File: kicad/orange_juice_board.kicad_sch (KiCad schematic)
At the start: 63 parts, among them J10 PWM_OUT1, J11 CONN_UART, J12 Conn_01x08, J12 PWM_OUT2, J13 FAN_12/24v, J15 PWM_OUT3, J2 DC_INPUT, J3 CONN_ADXL345, J4 OrangePi Zero GPIO PINs, J7 OrangePi Zero Function Interf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, J8 FAN_5v, J9 PWR_5v, Q1 AO4407A, Q2 AO3400A, Q3 AO3400A, Q4 AO3400A, U1 MP2315GJ-Z

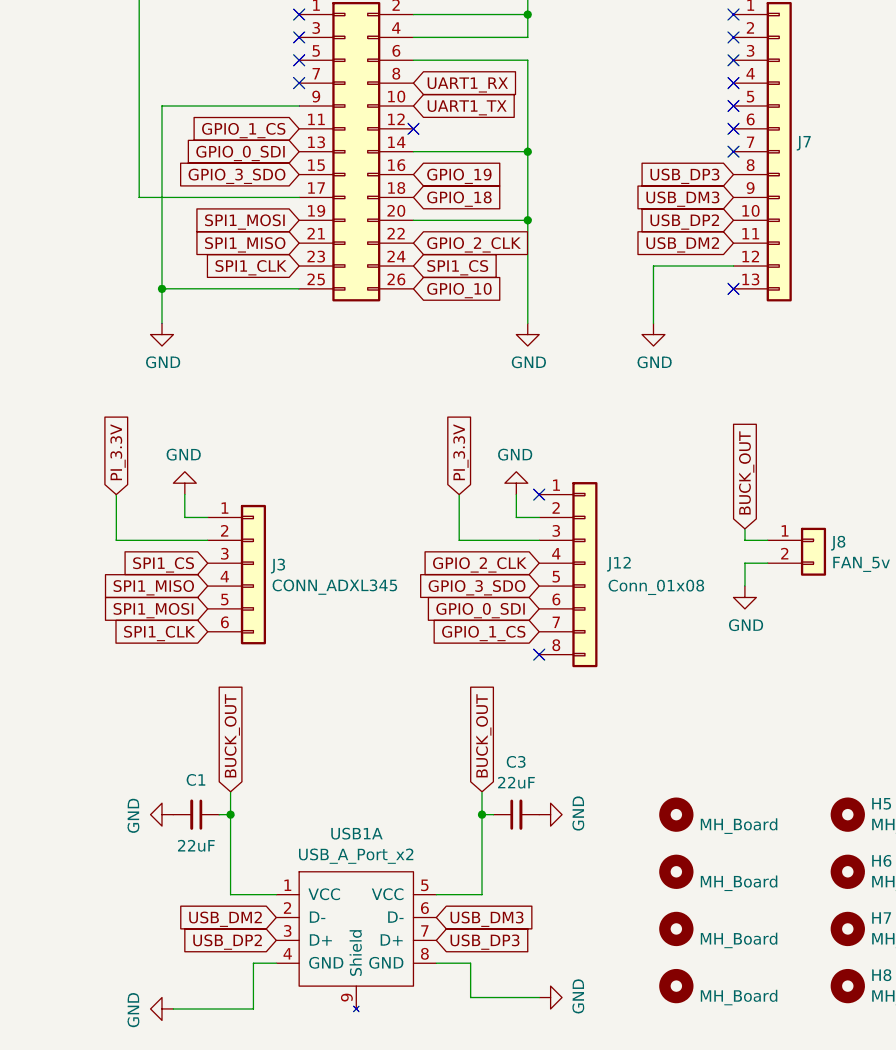
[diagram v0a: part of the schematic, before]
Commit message: update to v0.7
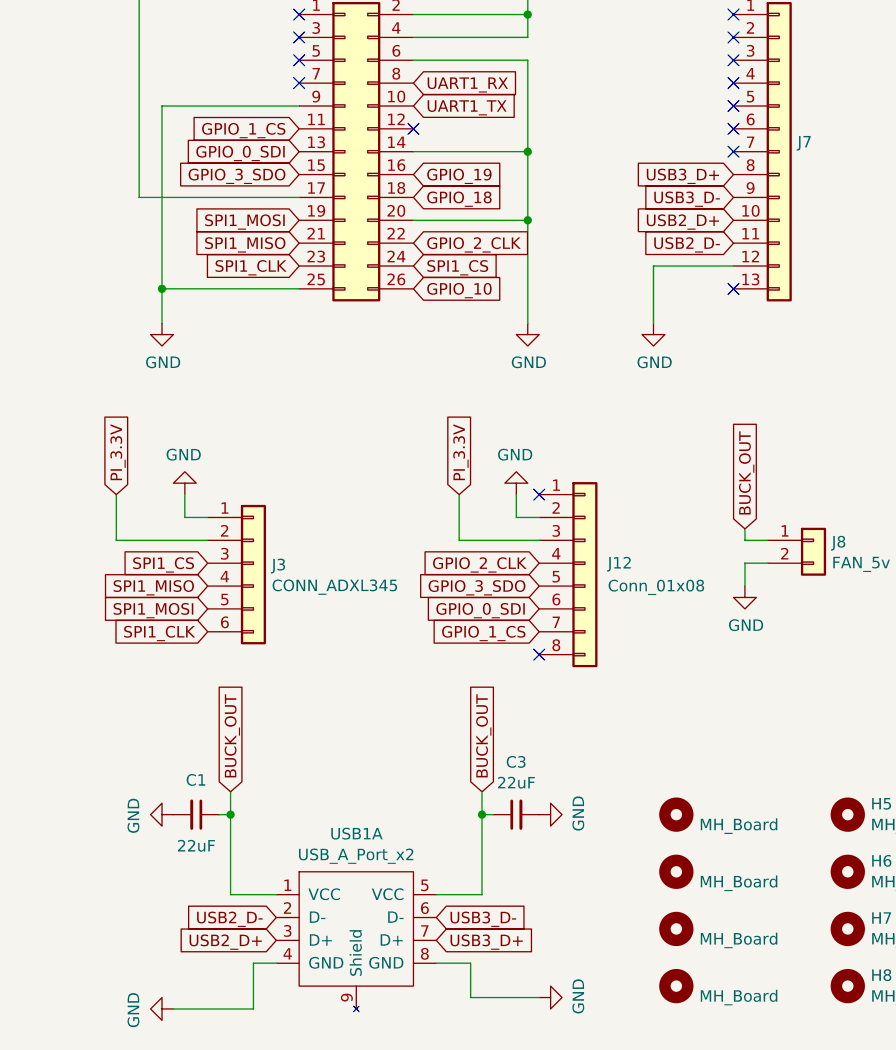
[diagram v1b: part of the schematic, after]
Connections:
- net USB_DM2 renamed USB2_D-
- net USB_DM3 renamed USB3_D-
- net USB_DP2 renamed USB2_D+
- net USB_DP3 renamed USB3_D+
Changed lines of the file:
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@@
     )
   )
-  (global_label "USB_DM2" (shape input) (at 95.25 101.6 180) (fields_autoplaced)
-    (effects (font (size 1.27 1.27)) (justify right))
-    (property "Intersheet References" "${INTERSHEET_REFS}" (id 0) (at -8.89 0 0)
-      (effects (font (size 1.27 1.27)) hide)
+  (global_label "USB2_D-" (shape input) (at 95.25 101.6 180) (fields_autoplaced)
+    (effects (font (size 1.27 1.27)) (justify right))
+    (property "Intersheet References" "${INTERSHEET_REFS}" (id 0) (at 84.0963 101.5206 0)
+      (effects (font (size 1.27 1.27)) (justify right) hide)
     )
   )
@@
     )
   )
-  (global_label "USB_DM3" (shape input) (at 62.23 176.53 0) (fields_autoplaced)
-    (effects (font (size 1.27 1.27)) (justify left))
-    (property "Intersheet References" "${INTERSHEET_REFS}" (id 0) (at 33.02 0 0)
-      (effects (font (size 1.27 1.27)) hide)
+  (global_label "USB3_D-" (shape input) (at 62.23 176.53 0) (fields_autoplaced)
+    (effects (font (size 1.27 1.27)) (justify left))
+    (property "Intersheet References" "${INTERSHEET_REFS}" (id 0) (at 73.3837 176.4506 0)
+      (effects (font (size 1.27 1.27)) (justify left) hide)
     )
   )
@@
     )
   )
-  (global_label "USB_DM2" (shape input) (at 44.45 176.53 180) (fields_autoplaced)
-    (effects (font (size 1.27 1.27)) (justify right))
-    (property "Intersheet References" "${INTERSHEET_REFS}" (id 0) (at 73.66 345.44 0)
-      (effects (font (size 1.27 1.27)) hide)
+  (global_label "USB2_D-" (shape input) (at 44.45 176.53 180) (fields_autoplaced)
+    (effects (font (size 1.27 1.27)) (justify right))
+    (property "Intersheet References" "${INTERSHEET_REFS}" (id 0) (at 33.2963 176.4506 0)
+      (effects (font (size 1.27 1.27)) (justify right) hide)
     )
   )
@@
     )
   )
-  (global_label "USB_DP2" (shape input) (at 44.45 179.07 180) (fields_autoplaced)
-    (effects (font (size 1.27 1.27)) (justify right))
-    (property "Intersheet References" "${INTERSHEET_REFS}" (id 0) (at 73.66 350.52 0)
-      (effects (font (size 1.27 1.27)) hide)
+  (global_label "USB2_D+" (shape input) (at 44.45 179.07 180) (fields_autoplaced)
+    (effects (font (size 1.27 1.27)) (justify right))
+    (property "Intersheet References" "${INTERSHEET_REFS}" (id 0) (at 33.2963 178.9906 0)
+      (effects (font (size 1.27 1.27)) (justify right) hide)
     )
   )
@@
     )
   )
-  (global_label "USB_DP2" (shape input) (at 95.25 99.06 180) (fields_autoplaced)
-    (effects (font (size 1.27 1.27)) (justify right))
-    (property "Intersheet References" "${INTERSHEET_REFS}" (id 0) (at -8.89 0 0)
-      (effects (font (size 1.27 1.27)) hide)
-    )
-  )
-  (global_label "USB_DP3" (shape input) (at 95.25 93.98 180) (fields_autoplaced)
-    (effects (font (size 1.27 1.27)) (justify right))
-    (property "Intersheet References" "${INTERSHEET_REFS}" (id 0) (at -8.89 0 0)
-      (effects (font (size 1.27 1.27)) hide)
+  (global_label "USB2_D+" (shape input) (at 95.25 99.06 180) (fields_autoplaced)
+    (effects (font (size 1.27 1.27)) (justify right))
+    (property "Intersheet References" "${INTERSHEET_REFS}" (id 0) (at 84.0963 98.9806 0)
+      (effects (font (size 1.27 1.27)) (justify right) hide)
+    )
+  )
+  (global_label "USB3_D+" (shape input) (at 95.25 93.98 180) (fields_autoplaced)
+    (effects (font (size 1.27 1.27)) (justify right))
+    (property "Intersheet References" "${INTERSHEET_REFS}" (id 0) (at 84.0963 93.9006 0)
+      (effects (font (size 1.27 1.27)) (justify right) hide)
     )
   )
@@
     )
   )
-  (global_label "USB_DM3" (shape input) (at 95.25 96.52 180) (fields_autoplaced)
-    (effects (font (size 1.27 1.27)) (justify right))
-    (property "Intersheet References" "${INTERSHEET_REFS}" (id 0) (at -8.89 0 0)
-      (effects (font (size 1.27 1.27)) hide)
+  (global_label "USB3_D-" (shape input) (at 95.25 96.52 180) (fields_autoplaced)
+    (effects (font (size 1.27 1.27)) (justify right))
+    (property "Intersheet References" "${INTERSHEET_REFS}" (id 0) (at 84.0963 96.4406 0)
+      (effects (font (size 1.27 1.27)) (justify right) hide)
     )
   )
@@
     )
   )
-  (global_label "USB_DP3" (shape input) (at 62.23 179.07 0) (fields_autoplaced)
-    (effects (font (size 1.27 1.27)) (justify left))
-    (property "Intersheet References" "${INTERSHEET_REFS}" (id 0) (at 33.02 0 0)
-      (effects (font (size 1.27 1.27)) hide)
-    )
-  )
+  (global_label "USB3_D+" (shape input) (at 62.23 179.07 0) (fields_autoplaced)
+    (effects (font (size 1.27 1.27)) (justify left))
+    (property "Intersheet References" "${INTERSHEET_REFS}" (id 0) (at 73.3837 178.9906 0)
+      (effects (font (size 1.27 1.27)) (justify left) hide)
+    )
+  )

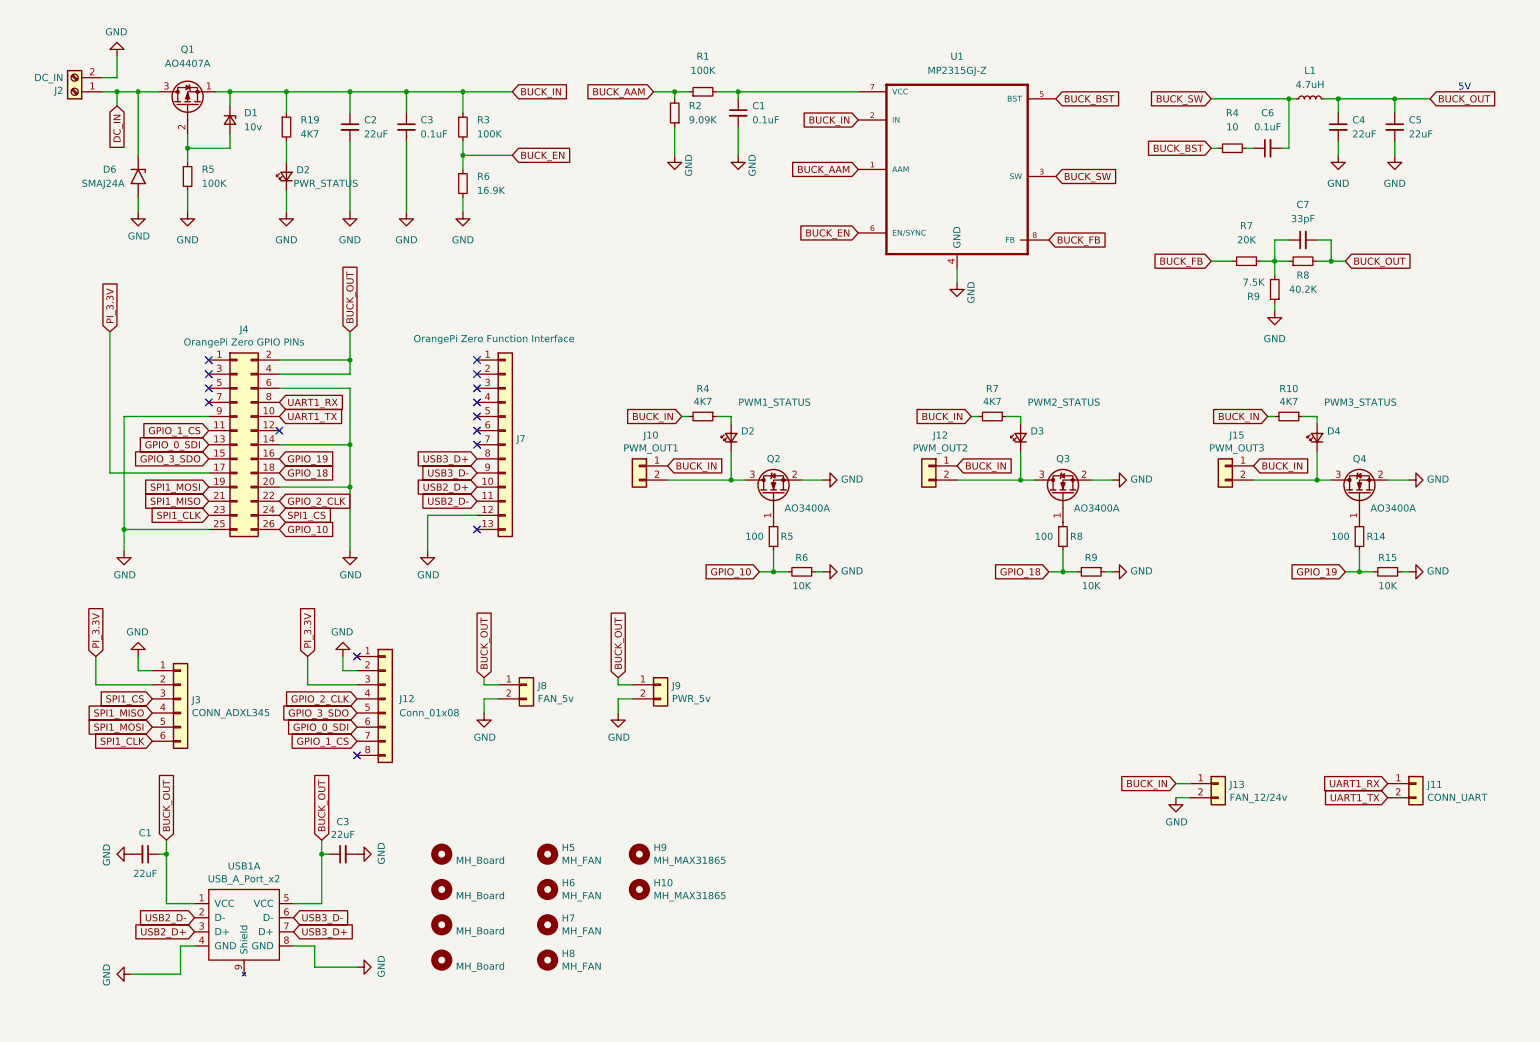
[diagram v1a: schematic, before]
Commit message: update to v0.7
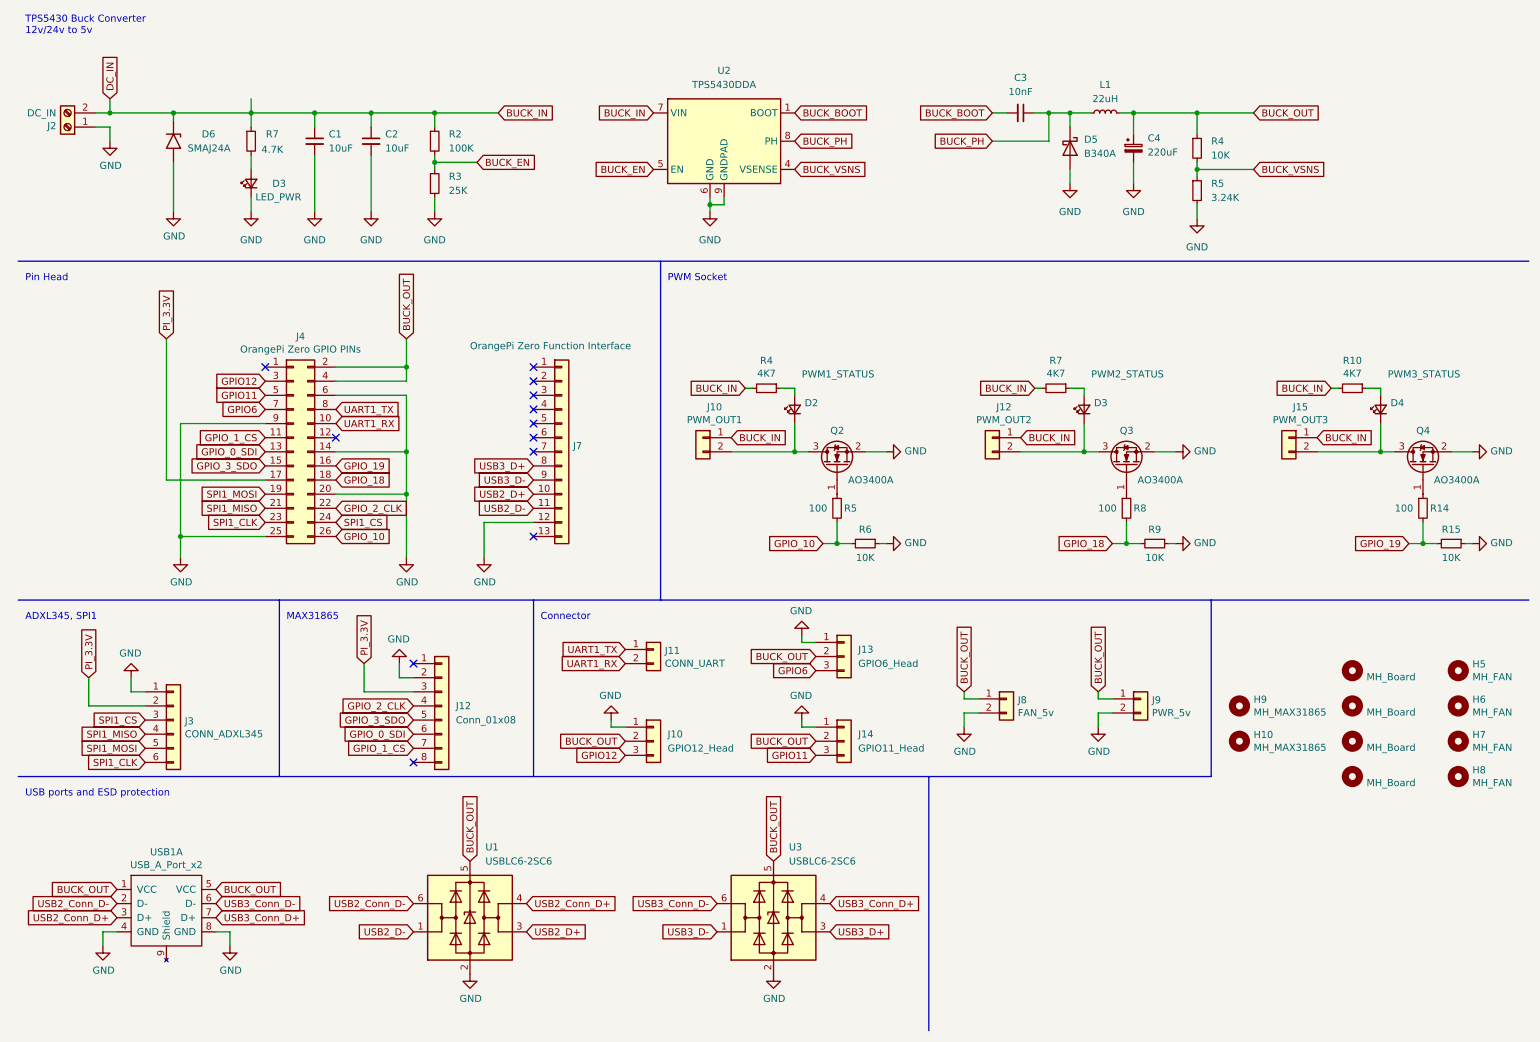
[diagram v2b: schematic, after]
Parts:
- removed C1, C3: 22u, Capacitor_SMD:C_0805_2012Metric, symbol orange_juice_board-rescue:C_Small-Device-OrangePiZeroExtentionBoard-rescue-oran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
- removed C4, C5: 22uF, Capacitor_SMD:C_0805_2012Metric, symbol Device:C_Small
- removed C6: 0.1uF, Capacitor_SMD:C_0805_2012Metric, symbol Device:C_Small
- removed C7: 33pF, Capacitor_SMD:C_0805_2012Metric, symbol Device:C_Small
- removed D1: 10v, Diode_SMD:D_SOD-123, symbol Device:D_Zener_Small
- removed D2: PWM1_STATUS, LED_SMD:LED_0805_2012Metric, symbol orange_juice_board-rescue:LED_Small-Device-OrangePiZeroExtentionBoard-rescue-or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
- removed J13: FAN_12/24v, Connector_JST:JST_XH_B2B-XH-A_1x02_P2.50mm_Vertical, symbol orange_juice_board-rescue:Conn_01x02-Connector_Generic-OrangePiZeroExtentionBoa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
- removed Q1: AO4407A, JerryLibrary:SOIC127P600X175-8N, symbol Device:Q_PMOS_SGD
- removed R1: 100K, Resistor_SMD:R_0805_2012Metric, symbol Device:R_Small
- removed R19: 4K7, Resistor_SMD:R_0805_2012Metric, symbol Device:R_Small
- removed R6: 16.9K, Resistor_SMD:R_0805_2012Metric, symbol Device:R_Small
- removed R7: 20K, Resistor_SMD:R_0805_2012Metric, symbol Device:R_Small
- removed R8: 40.2K, Resistor_SMD:R_0805_2012Metric, symbol Device:R_Small
- removed R9: 7.5K, Resistor_SMD:R_0805_2012Metric, symbol Device:R_Small
- removed U1: MP2315GJ-Z, Package_TO_SOT_SMD:SOT-23-8, symbol Jerry_Library:MP2315GJ-Z
- added C4: 220uF, Capacitor_SMD:C_Elec_6.3x5.4, symbol Device:C_Polarized_Small
- added D3: PWM2_STATUS, LED_SMD:LED_0805_2012Metric, symbol orange_juice_board-rescue:LED_Small-Device-OrangePiZeroExtentionBoard-rescue-or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
- added D5: B340A, Diode_SMD:D_SMA, symbol Diode:B340
- added J10: GPIO12_Head, Connector_PinHeader_2.54mm:PinHeader_1x03_P2.54mm_Vertical, symbol Connector_Generic:Conn_01x03
- added J13: GPIO6_Head, Connector_PinHeader_2.54mm:PinHeader_1x03_P2.54mm_Vertical, symbol Connector_Generic:Conn_01x03
- added J14: GPIO11_Head, Connector_PinHeader_2.54mm:PinHeader_1x03_P2.54mm_Vertical, symbol Connector_Generic:Conn_01x03
- added R7: 4k7, Resistor_SMD:R_0805_2012Metric, symbol orange_juice_board-rescue:R_Small-Device-OrangePiZeroExtentionBoard-rescue-oran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
- added U1, U3: USBLC6-2SC6, Package_TO_SOT_SMD:SOT-23-6, symbol Power_Protection:USBLC6-2SC6
- added U2: TPS5430DDA, Package_SO:TI_SO-PowerPAD-8_ThermalVias, symbol Regulator_Switching:TPS5430DDA
- C1: value 0.1uF -> 10uF; footprint Capacitor_SMD:C_0805_2012Metric -> Capacitor_SMD:C_1206_3216Metric; LCSC Part# C49678 -> (none)
- C2: value 22uF -> 10uF; LCSC Part# C2835562 -> (none)
- C3: value 0.1uF -> 10nF; LCSC Part# C49678 -> (none)
- D6: footprint Diode_SMD:D_SMB -> Diode_SMD:D_SMA
- L1: value 4.7uH -> 22uH; footprint Inductor_SMD:L_Abracon_ASPI-0630LR -> Inductor_SMD:L_7.3x7.3_H4.5; LCSC Part# C128688 -> (none)
- R2: value 9.09K -> 100K; LCSC Part# C17854 -> (none)
- R3: value 100K -> 25K; LCSC Part# C96346 -> (none)
- R4: value 10 -> 10K; LCSC Part# C17415 -> (none)
- R5: value 100K -> 3.24K; LCSC Part# C96346 -> (none)
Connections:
- net BUCK_AAM is gone; now on net BUCK_EN: R2.2
- net BUCK_BST is gone; now on net BUCK_OUT: R4.1
- net BUCK_EN: now also R3.1, U2.5 (EN); no longer R3.2
- net BUCK_IN: now also C1.1, D6.1 (A1), J2.2 (Pin_2), R2.1, R7.1, U2.7 (VIN); no longer C3.1, R3.1
- net BUCK_OUT: now also C4.1, J10.2 (Pin_2), J13.2 (Pin_2), J14.2 (Pin_2), U1.5 (VBUS), U3.5 (VBUS)
- net GND: now also J2.1 (Pin_1), R3.2, C4.2, D3.1 (K), D5.2 (A), J10.1 (Pin_1), J13.1 (Pin_1), J14.1 (Pin_1), U1.2 (GND), U2.6 (GND), U2.9 (GNDPAD), U3.2 (GND); no longer C3.2, J2.2 (Pin_2), R2.1
- net UART1_RX: now also J11.2 (Pin_2), J4.10 (Pin_10); no longer J11.1 (Pin_1), J4.8 (Pin_8)
- net UART1_TX: now also J11.1 (Pin_1), J4.8 (Pin_8); no longer J11.2 (Pin_2), J4.10 (Pin_10)
- net USB2_D+: now also U1.3 (I/O2); no longer USB1.3 (D+)
- net USB2_D-: now also U1.1 (I/O1); no longer USB1.2 (D-)
- net USB3_D+: now also U3.3 (I/O2); no longer USB1.7 (D+)
- net USB3_D-: now also U3.1 (I/O1); no longer USB1.6 (D-)
- net GPIO12: now reaches J4.3 (Pin_3)
- net GPIO12: now also J10.3 (Pin_3)
- net GPIO11: now reaches J4.5 (Pin_5)
- net GPIO11: now also J14.3 (Pin_3)
- net GPIO6: now reaches J4.7 (Pin_7)
- net GPIO6: now also J13.3 (Pin_3)
- net BUCK_VSNS: now reaches R4.2
- net BUCK_VSNS: now also R5.1, U2.4 (VSENSE)
- net BUCK_SW renamed BUCK_PH
- net BUCK_PH: now also C3.1, D5.1 (K), U2.8 (PH)
- removed net DC_IN: D6.1 (A1), J2.1 (Pin_1)
- new net: D3.2 (A), R7.2
- new net BUCK_BOOT: C3.2, U2.1 (BOOT)
- new net USB2_Conn_D+: U1.4 (I/O2), USB1.3 (D+)
- new net USB2_Conn_D-: U1.6 (I/O1), USB1.2 (D-)
- new net USB3_Conn_D+: U3.4 (I/O2), USB1.7 (D+)
- new net USB3_Conn_D-: U3.6 (I/O1), USB1.6 (D-)
- no-connect marks 15 -> 12
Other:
- note added: "ADXL345, SPI1"
- note added: "Connector"
- note added: "MAX31865"
- note added: "PWM Socket"
- note added: "Pin Head"
- note added: "TPS5430 Buck Converter 12v/24v to 5v"
- note added: "USB ports and ESD protection"
- note removed: "5V"
- moved on the sheet: D2, D3, D4, D6, H10, H5, H6, H7, H8, H9, J10, J11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
